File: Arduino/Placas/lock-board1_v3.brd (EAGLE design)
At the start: 174.5 x 106.5 mm, 18 parts

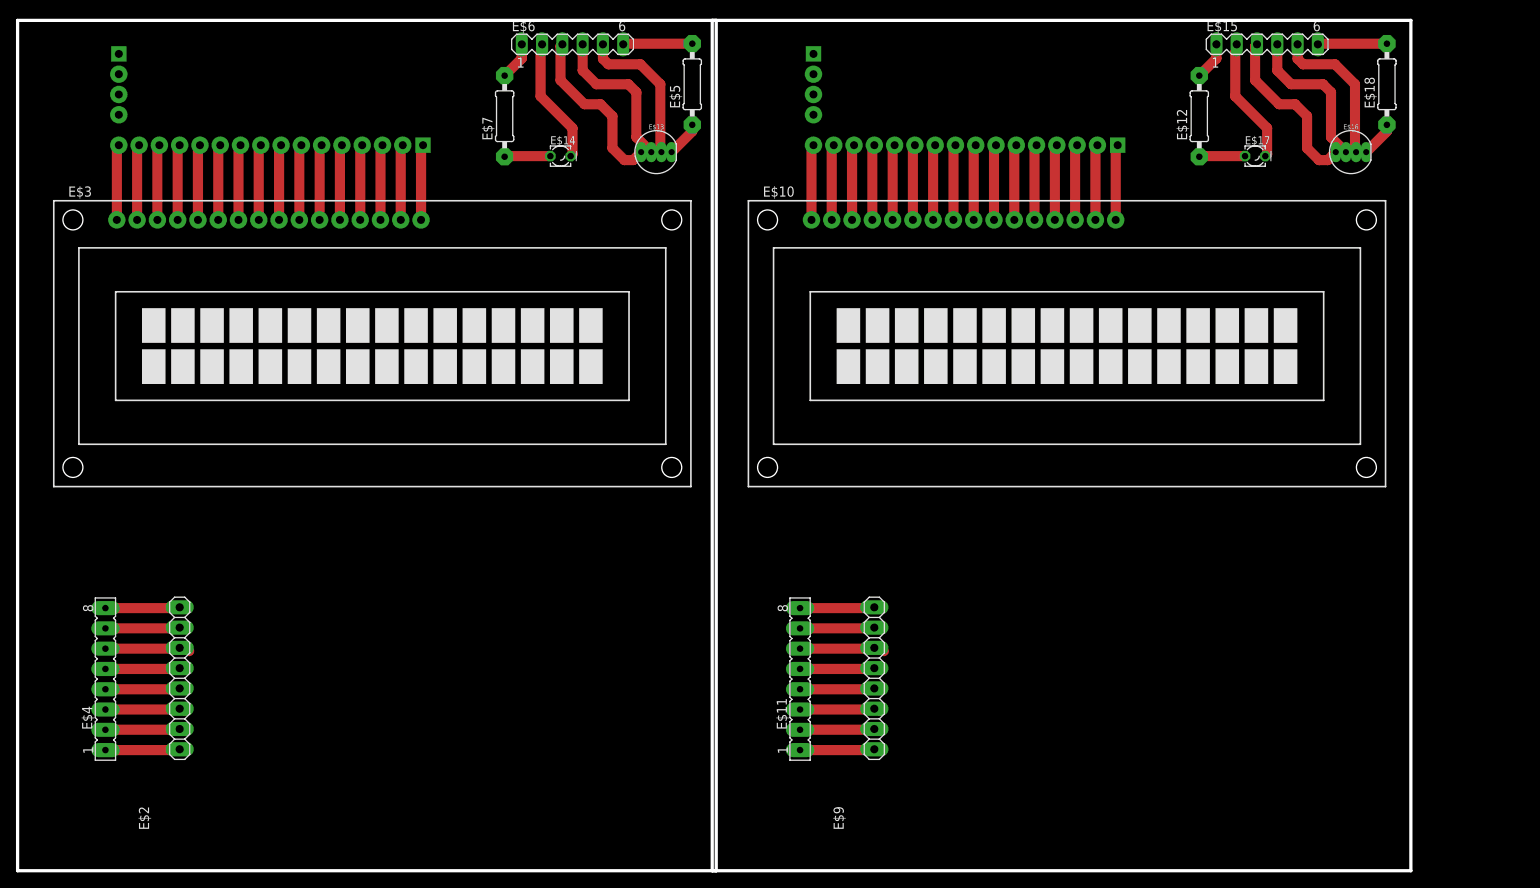
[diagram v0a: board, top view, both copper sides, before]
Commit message: Lock board updated
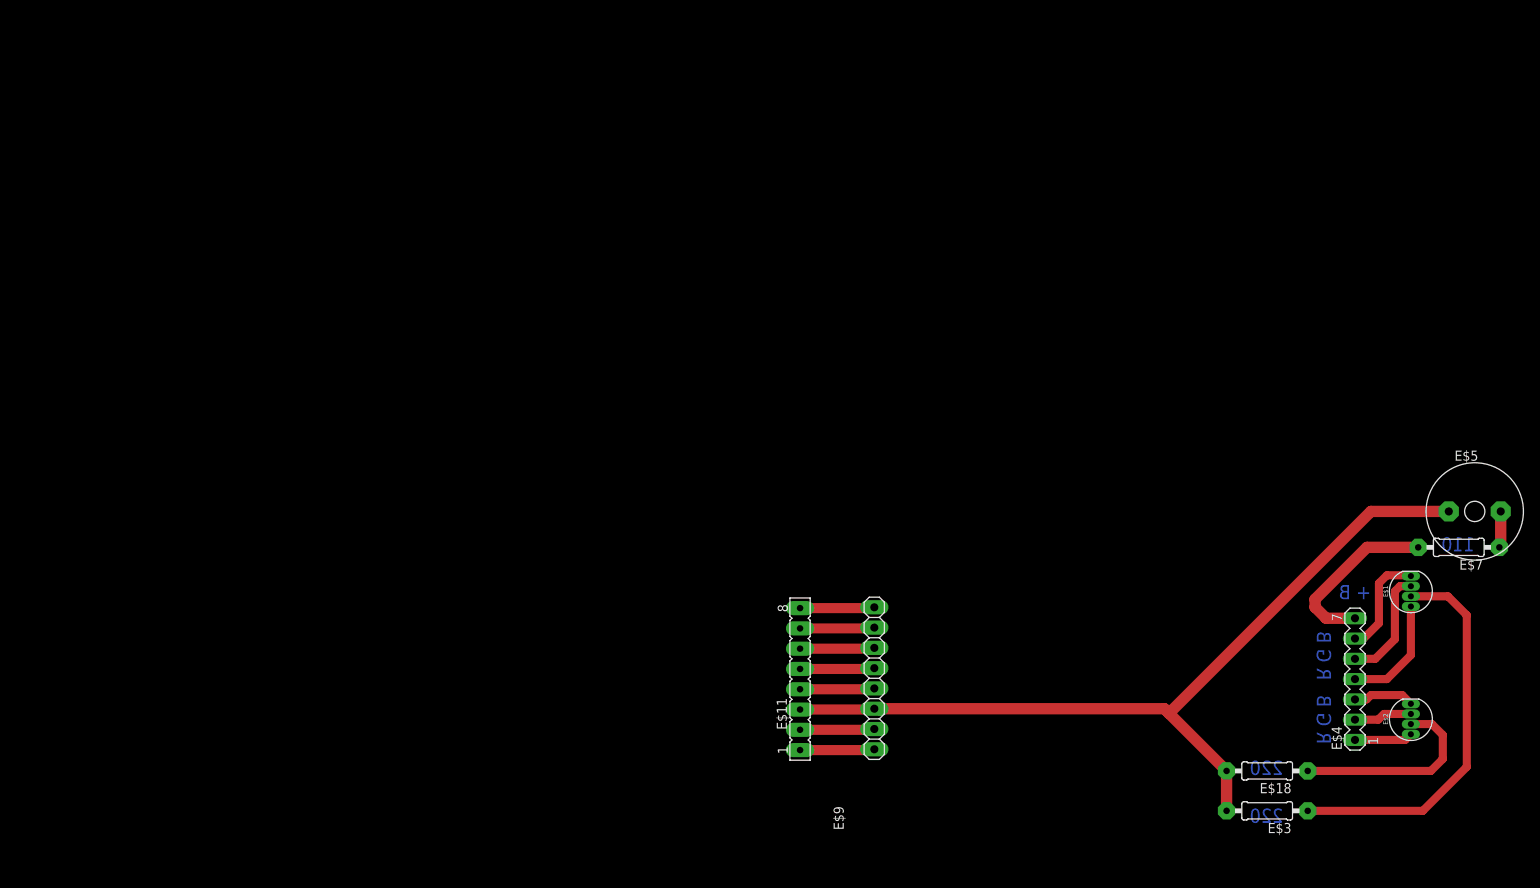
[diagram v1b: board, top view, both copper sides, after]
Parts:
- removed E$10: (no value), display-lcd:TUXGR_16X2_R2
- removed E$12: (no value), eagle-ltspice:0207/10
- removed E$13, E$16: (no value), SparkFun-LED:LED-RGB-THRU
- removed E$14, E$17: (no value), eagle-ltspice:LED_LD260
- removed E$15, E$6: (no value), con-lstb:MA06-1
- removed E$8: (no value), converter_lcd_serial_i2c:LCD-I2C-CONVERTER
- E$1: device converter_lcd_serial_i2c:LCD-I2C-CONVERTER -> SparkFun-LED:LED-RGB-THRU
- E$2: device mfrc522-module:RFID-RC522 -> SparkFun-LED:LED-RGB-THRU
- E$3: device display-lcd:TUXGR_16X2_R2 -> eagle-ltspice:0207/10
- E$4: device con-lsta:FE08 -> con-lstb:MA07-1
- E$5: device eagle-ltspice:0207/10 -> buzzer:AL60P
- moved E$4 156.5 mm to (198.0, 38.0)
- moved E$1 155.7 mm to (205.0, 49.0), flipped to the top, turned to 90 degrees
- moved E$2 154.3 mm to (205.0, 33.0)
- moved E$7 131.1 mm to (211.0, 54.5), turned to 180 degrees
- moved E$3 126.4 mm to (187.0, 21.5), turned to 180 degrees
- moved E$5 111.7 mm to (213.0, 59.0), turned to 0 degrees
- moved E$18 87.3 mm to (187.0, 26.5), turned to 180 degrees
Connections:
- removed net S$14: E$1.J2.2, E$3.15
- removed net S$15: E$1.J2.1, E$3.16
- removed net S$16: E$1.J2.5, E$3.12
- removed net S$17: E$2.SS, E$4.8
- removed net S$18: E$2.SCK, E$4.7
- removed net S$19: E$2.MOSI, E$4.6
- removed net S$2: E$1.J2.15, E$3.2
- removed net S$20: E$2.MISO, E$4.5
- removed net S$21: E$4.4
- removed net S$22: E$2.GND, E$4.3
- removed net S$23: E$2.RST, E$4.2
- removed net S$24: E$2.3V3, E$4.1
- removed net S$25: E$2.IRQ
- removed net S$26: E$1.J2.6, E$3.11
- removed net S$27: E$6.1, E$7.2
- removed net S$28: E$5.2, E$6.6
- removed net S$29: E$13.1, E$5.1
- removed net S$30: E$13.2, E$6.5
- removed net S$31: E$13.3, E$6.4
- removed net S$32: E$13.4, E$6.3
- removed net S$33: E$14.K, E$6.2
- removed net S$34: E$10.1, E$8.J2.16
- removed net S$35: E$10.2, E$8.J2.15
- removed net S$36: E$10.3, E$8.J2.14
- removed net S$37: E$10.4, E$8.J2.13
- removed net S$38: E$10.5, E$8.J2.12
- removed net S$39: E$10.6, E$8.J2.11
- removed net S$40: E$10.7, E$8.J2.10
- removed net S$41: E$10.8, E$8.J2.9
- removed net S$42: E$10.9, E$8.J2.8
- removed net S$43: E$10.10, E$8.J2.7
- removed net S$44: E$10.11, E$8.J2.6
- removed net S$45: E$10.13, E$8.J2.4
- removed net S$46: E$10.14, E$8.J2.3
- removed net S$47: E$10.15, E$8.J2.2
- removed net S$48: E$10.16, E$8.J2.1
- removed net S$49: E$10.12, E$8.J2.5
- removed net S$5: E$1.J2.12, E$3.5
- removed net S$59: E$12.1, E$17.A
- removed net S$60: E$15.6, E$18.2
- removed net S$61: E$12.2, E$15.1
- removed net S$62: E$16.1, E$18.1
- removed net S$63: E$15.5, E$16.2
- removed net S$64: E$15.4, E$16.3
- removed net S$65: E$15.3, E$16.4
- removed net S$66: E$15.2, E$17.K
- removed net S$9: E$1.J2.8, E$3.9
- net S$1: now also E$18.1, E$2.3; no longer E$1.J2.16, E$3.1
- net S$10: now also E$2.1, E$4.3; no longer E$1.J2.7, E$3.10
- net S$11: now also E$1.4, E$4.4; no longer E$14.A, E$7.1
- net S$12: now also E$1.2, E$4.5; no longer E$1.J2.4, E$3.13
- net S$13: now also E$1.1, E$4.6; no longer E$1.J2.3, E$3.14
- net S$3: now also E$1.3, E$3.1; no longer E$1.J2.14, E$3.3
- net S$4: now also E$2.4, E$4.1; no longer E$1.J2.13, E$3.4
- net S$52: no longer E$9.MOSI
- net S$56: now also E$18.2, E$3.2, E$5.1
- net S$6: now also E$4.7, E$7.2; no longer E$1.J2.11, E$3.6
- net S$7: now also E$5.2, E$7.1; no longer E$1.J2.10, E$3.7
- net S$8: now also E$2.2, E$4.2; no longer E$1.J2.9, E$3.8
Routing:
- net S$56: track 10.1 -> 107.9 mm
- net S$3: track 9.46 -> 49.2 mm
- net S$32: track 21.6 -> 0.00 mm
- net S$65: track 21.6 -> 0.00 mm
- net S$64: track 19.4 -> 0.00 mm
- net S$31: track 19.4 -> 0.00 mm
- net S$30: track 18.9 -> 0.00 mm
- net S$63: track 18.9 -> 0.00 mm
- net S$33: track 15.8 -> 0.00 mm
- net S$66: track 15.8 -> 0.00 mm
- net S$1: track 9.46 -> 25.1 mm
- net S$6: track 9.46 -> 22.2 mm
- net S$19: track 10.6 -> 0.00 mm
- net S$22: track 10.1 -> 0.00 mm
- net S$23: track 10.1 -> 0.00 mm
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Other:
- board outline removed
- board text added: "+ B"
- board text added: "110"
- board text added: "220"
- board text added: "R G B"
